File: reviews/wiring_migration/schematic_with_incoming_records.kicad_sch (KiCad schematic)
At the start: 62 parts, among them J1 T4171310004-001, J2 3PH-4W-PLUG, J3 BNSPDX-23-W, J4 BSPDX-23-W, J5 BSPBX-22-W, K1 HMC-9B30-11-DS, K2 HMC-9B30-11-DS, K3 HC3096N-52-900-24, K4 HMC-9B30-11-DS, K5 HMC-9B30-11-DS, K6 HMC-9B30-11-DS, M1 PWRM1200-MOTOR, Q1 FAZ-D4/2-NA-L, SW1 222102

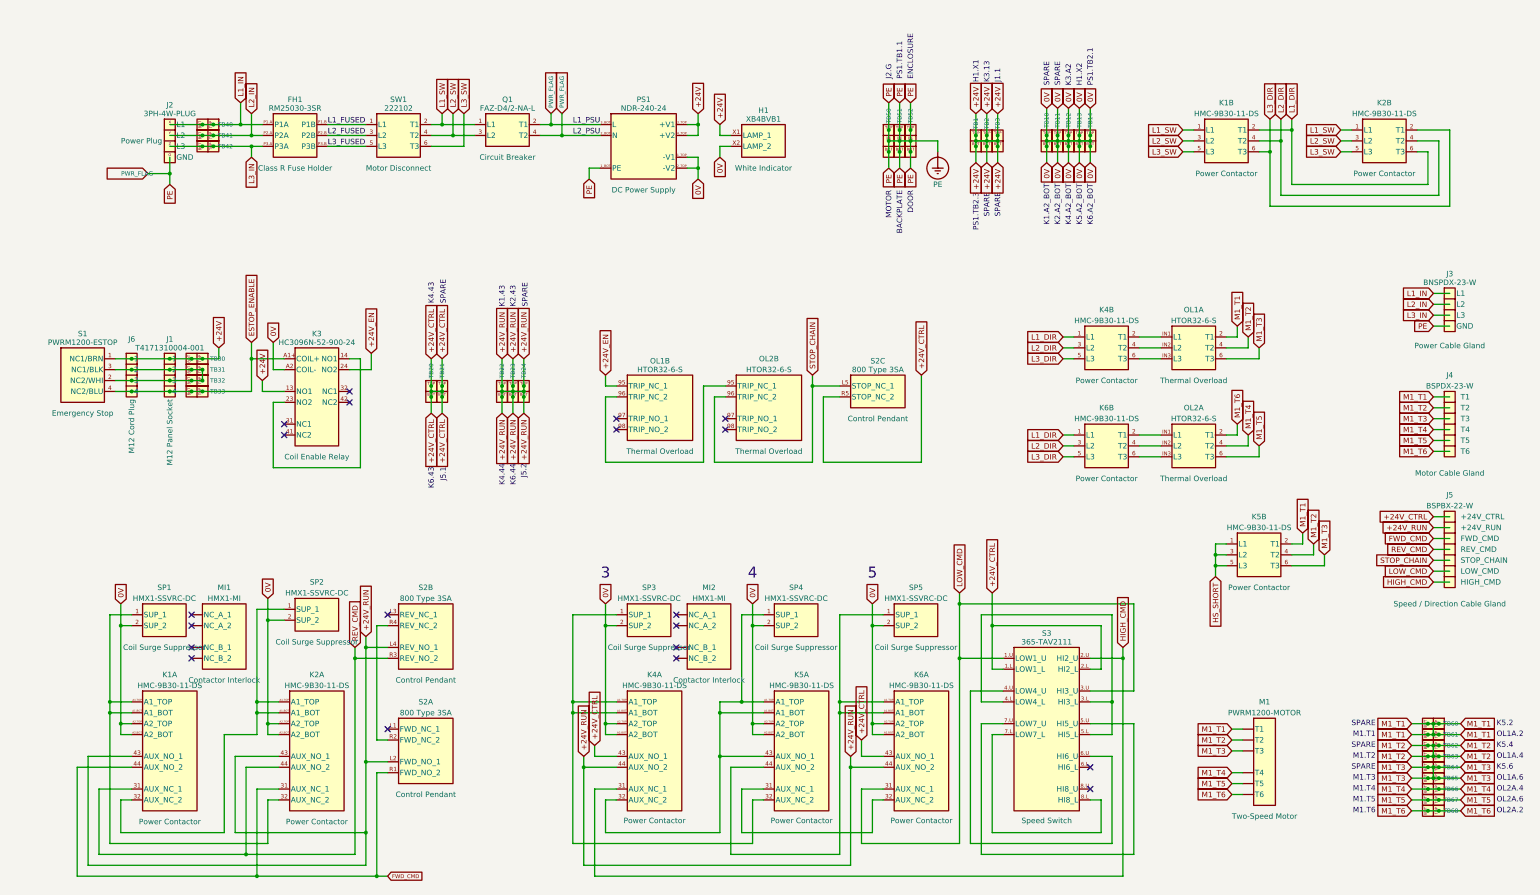
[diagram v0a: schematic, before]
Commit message: terminal block wiring
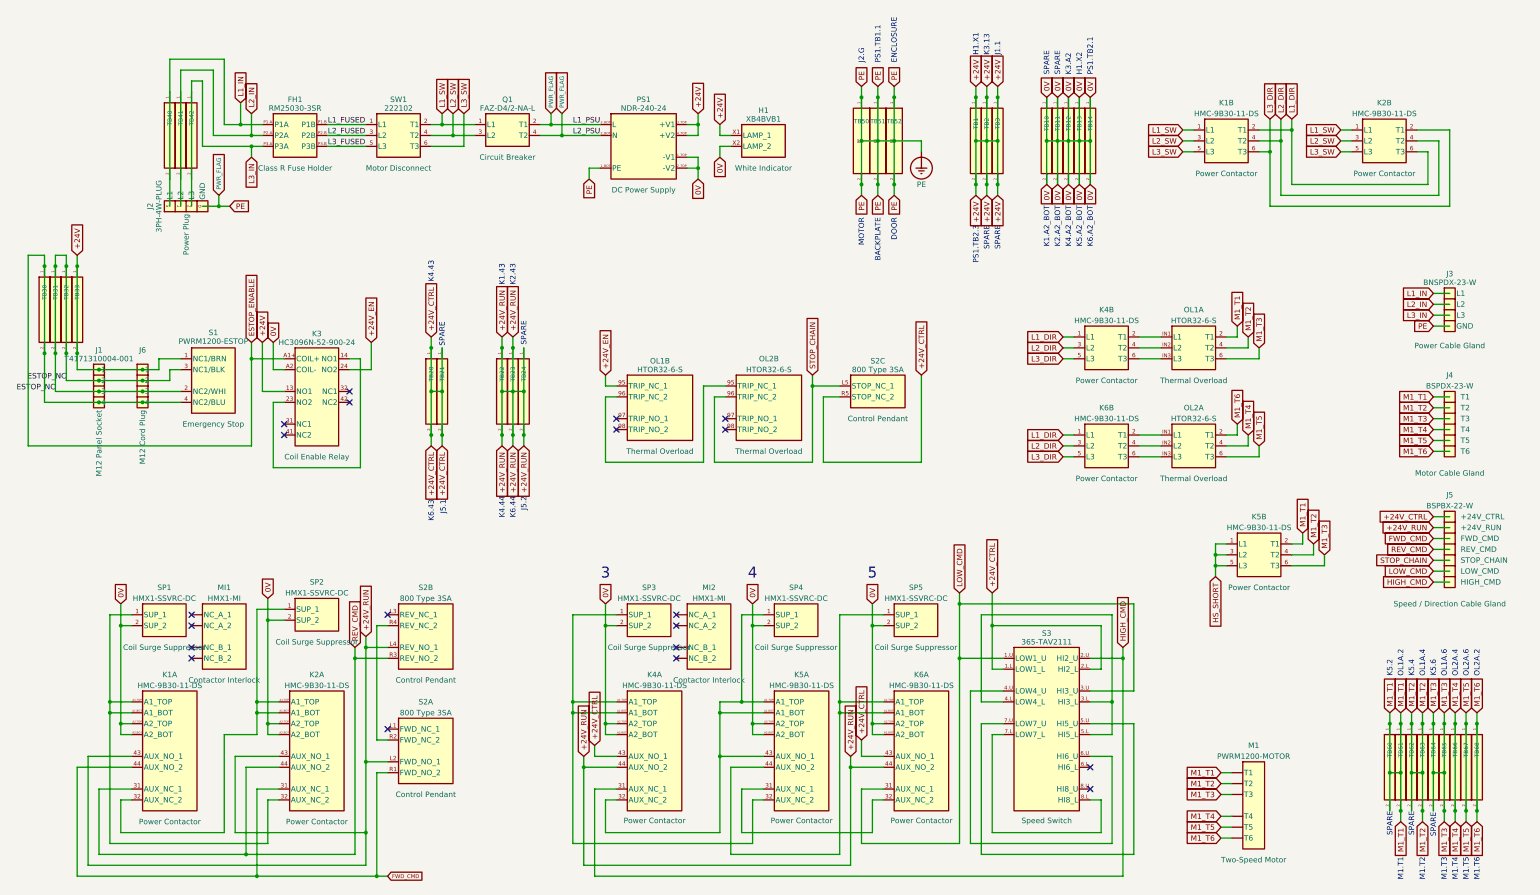
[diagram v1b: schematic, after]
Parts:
- J2: Wire.W001 {"schema":1,"from_pin":"X","to":{"symbol_uuid":"782cabbe-a58e-46f3-9f97-d5cf96f2f77e","pin":"BOT"},"section":"01 Incoming phases","kind":"panel_cable_core","review":"pending","awg":"12","term1":"plug clamp","term2":"Ferrule 12 AWG; L=TBD mm","length":{"mode":"auto","slack_mm":"200","round_mm":"50","minimum_mm":"400"},"migration_note":"The legacy cut estimate is retained as a minimum until this section is reviewed. Length covers the panel tail; external cable allowance remains in the BOM.","route_from":{"symbol_uuid":"233d10ed-562b-4d7c-8332-858e4146f140","pin":"X"},"from_symbol_uuid":"c5ff8006-339f-4474-94f3-df6cc7c1d5be"} -> {"schema":1,"from_pin":"X","to":{"symbol_uuid":"782cabbe-a58e-46f3-9f97-d5cf96f2f77e","pin":"2"},"section":"01 Incoming phases","kind":"panel_cable_core","review":"pending","awg":"12","term1":"plug clamp","term2":"Ferrule 12 AWG; L=TBD mm","length":{"mode":"auto","slack_mm":"200","round_mm":"50","minimum_mm":"400"},"migration_note":"The legacy cut estimate is retained as a minimum until this section is reviewed. Length covers the panel tail; external cable allowance remains in the BOM.","route_from":{"symbol_uuid":"233d10ed-562b-4d7c-8332-858e4146f140","pin":"X"}}; Wire.W003 {"schema":1,"from_pin":"Y","to":{"symbol_uuid":"28685e83-b92d-43bf-876f-d867e00acc25","pin":"BOT"},"section":"01 Incoming phases","kind":"panel_cable_core","review":"pending","awg":"12","term1":"plug clamp","term2":"Ferrule 12 AWG; L=TBD mm","length":{"mode":"auto","slack_mm":"200","round_mm":"50","minimum_mm":"400"},"migration_note":"The legacy cut estimate is retained as a minimum until this section is reviewed. Length covers the panel tail; external cable allowance remains in the BOM.","route_from":{"symbol_uuid":"233d10ed-562b-4d7c-8332-858e4146f140","pin":"Y"},"from_symbol_uuid":"c5ff8006-339f-4474-94f3-df6cc7c1d5be"} -> {"schema":1,"from_pin":"Y","to":{"symbol_uuid":"28685e83-b92d-43bf-876f-d867e00acc25","pin":"2"},"section":"01 Incoming phases","kind":"panel_cable_core","review":"pending","awg":"12","term1":"plug clamp","term2":"Ferrule 12 AWG; L=TBD mm","length":{"mode":"auto","slack_mm":"200","round_mm":"50","minimum_mm":"400"},"migration_note":"The legacy cut estimate is retained as a minimum until this section is reviewed. Length covers the panel tail; external cable allowance remains in the BOM.","route_from":{"symbol_uuid":"233d10ed-562b-4d7c-8332-858e4146f140","pin":"Y"}}; Wire.W005 {"schema":1,"from_pin":"Z","to":{"symbol_uuid":"d4d821a2-498b-4b0e-b253-9376599824db","pin":"BOT"},"section":"01 Incoming phases","kind":"panel_cable_core","review":"pending","awg":"12","term1":"plug clamp","term2":"Ferrule 12 AWG; L=TBD mm","length":{"mode":"auto","slack_mm":"200","round_mm":"50","minimum_mm":"400"},"migration_note":"The legacy cut estimate is retained as a minimum until this section is reviewed. Length covers the panel tail; external cable allowance remains in the BOM.","route_from":{"symbol_uuid":"233d10ed-562b-4d7c-8332-858e4146f140","pin":"Z"},"from_symbol_uuid":"c5ff8006-339f-4474-94f3-df6cc7c1d5be"} -> {"schema":1,"from_pin":"Z","to":{"symbol_uuid":"d4d821a2-498b-4b0e-b253-9376599824db","pin":"2"},"section":"01 Incoming phases","kind":"panel_cable_core","review":"pending","awg":"12","term1":"plug clamp","term2":"Ferrule 12 AWG; L=TBD mm","length":{"mode":"auto","slack_mm":"200","round_mm":"50","minimum_mm":"400"},"migration_note":"The legacy cut estimate is retained as a minimum until this section is reviewed. Length covers the panel tail; external cable allowance remains in the BOM.","route_from":{"symbol_uuid":"233d10ed-562b-4d7c-8332-858e4146f140","pin":"Z"}}
- TB40: Wire.W002 {"schema":1,"from_pin":"TOP","to":{"symbol_uuid":"5ca8057b-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 -> {"schema":1,"from_pin":"1","to":{"symbol_uuid":"5ca8057b-4e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
- TB41: Wire.W004 {"schema":1,"from_pin":"TOP","to":{"symbol_uuid":"5ca8057b-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 -> {"schema":1,"from_pin":"1","to":{"symbol_uuid":"5ca8057b-4e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
- TB42: Wire.W006 {"schema":1,"from_pin":"TOP","to":{"symbol_uuid":"5ca8057b-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 -> {"schema":1,"from_pin":"1","to":{"symbol_uuid":"5ca8057b-4e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
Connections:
- net +24V: now also TB1.1 (TERM), TB1.2 (TERM), TB2.1 (TERM), TB2.2 (TERM), TB3.1 (TERM), TB3.2 (TERM), TB33.1 (TERM), TB33.2 (TERM); no longer TB1.BOT (TERM), TB1.TOP (TERM), TB2.BOT (TERM), TB2.TOP (TERM), TB3.BOT (TERM), TB3.TOP (TERM), TB30.BOT (TERM), TB30.TOP (TERM)
- net +24V_CTRL: now also TB20.1 (TERM), TB20.2 (TERM), TB21.1 (TERM), TB21.2 (TERM); no longer TB20.BOT (TERM), TB20.TOP (TERM), TB21.BOT (TERM), TB21.TOP (TERM)
- net +24V_RUN: now also TB22.1 (TERM), TB22.2 (TERM), TB23.1 (TERM), TB23.2 (TERM), TB24.1 (TERM), TB24.2 (TERM); no longer TB22.BOT (TERM), TB22.TOP (TERM), TB23.BOT (TERM), TB23.TOP (TERM), TB24.BOT (TERM), TB24.TOP (TERM)
- net 0V: now also TB10.1 (TERM), TB10.2 (TERM), TB11.1 (TERM), TB11.2 (TERM), TB12.1 (TERM), TB12.2 (TERM), TB13.1 (TERM), TB13.2 (TERM), TB14.1 (TERM), TB14.2 (TERM); no longer TB10.BOT (TERM), TB10.TOP (TERM), TB11.BOT (TERM), TB11.TOP (TERM), TB12.BOT (TERM), TB12.TOP (TERM), TB13.BOT (TERM), TB13.TOP (TERM), TB14.BOT (TERM), TB14.TOP (TERM)
- net ESTOP_ENABLE: now also TB30.1 (TERM), TB30.2 (TERM); no longer TB33.BOT (TERM), TB33.TOP (TERM)
- net L1_IN: now also TB40.1 (TERM), TB40.2 (TERM); no longer TB40.BOT (TERM), TB40.TOP (TERM)
- net L2_IN: now also TB41.1 (TERM), TB41.2 (TERM); no longer TB41.BOT (TERM), TB41.TOP (TERM)
- net L3_IN: now also TB42.1 (TERM), TB42.2 (TERM); no longer TB42.BOT (TERM), TB42.TOP (TERM)
- net M1_T1: now also TB60.1 (TERM), TB60.2 (TERM), TB61.1 (TERM), TB61.2 (TERM); no longer TB60.BOT (TERM), TB60.TOP (TERM), TB61.BOT (TERM), TB61.TOP (TERM)
- net M1_T2: now also TB62.1 (TERM), TB62.2 (TERM), TB63.1 (TERM), TB63.2 (TERM); no longer TB62.BOT (TERM), TB62.TOP (TERM), TB63.BOT (TERM), TB63.TOP (TERM)
- net M1_T3: now also TB64.1 (TERM), TB64.2 (TERM), TB65.1 (TERM), TB65.2 (TERM); no longer TB64.BOT (TERM), TB64.TOP (TERM), TB65.BOT (TERM), TB65.TOP (TERM)
- net M1_T4: now also TB66.1 (TERM), TB66.2 (TERM); no longer TB66.BOT (TERM), TB66.TOP (TERM)
- net M1_T5: now also TB67.1 (TERM), TB67.2 (TERM); no longer TB67.BOT (TERM), TB67.TOP (TERM)
- net M1_T6: now also TB68.1 (TERM), TB68.2 (TERM); no longer TB68.BOT (TERM), TB68.TOP (TERM)
- net PE: now also TB50.1 (TERM), TB50.2 (TERM), TB51.1 (TERM), TB51.2 (TERM), TB52.1 (TERM), TB52.2 (TERM); no longer TB50.BOT (TERM), TB50.TOP (TERM), TB51.BOT (TERM), TB51.TOP (TERM), TB52.BOT (TERM), TB52.TOP (TERM)
- net ESTOP_NC: now reaches J1.2, J1.3, J6.2, J6.3, S1.2 (NC2/WHI), S1.3 (NC1/BLK)
- net ESTOP_NC: now also TB31.1 (TERM), TB31.2 (TERM), TB32.1 (TERM), TB32.2 (TERM); no longer TB31.BOT (TERM), TB31.TOP (TERM), TB32.BOT (TERM), TB32.TOP (TERM)
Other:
- moved on the sheet: M1, TB50, TB51, TB52
